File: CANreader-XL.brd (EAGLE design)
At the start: 99.8 x 49.8 mm, 101 parts, among them IC1 STM32F107RBT, IC2 TJA1055T/3, IC3 BD9G101G, IC4 LM1117IMPX-3.3, IC5 MCP2562-SOIC8, IC7 DP83848I, Q1 25MHz, SW1 SLEEP, SW2 TERM, U1 HC_05, X1 ST-USB-009A, X2 SWD, X3 CAN+GPIO, X4 UART

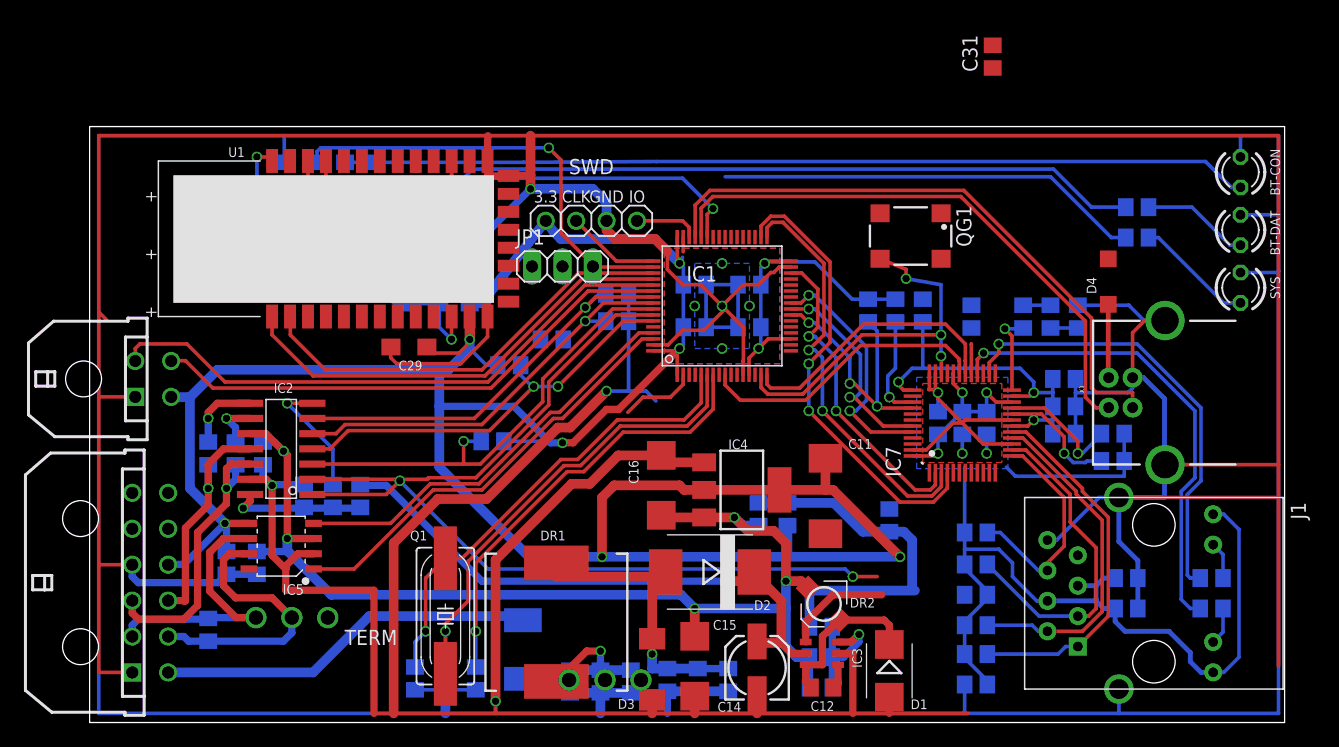
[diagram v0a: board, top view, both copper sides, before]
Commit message: Route attempt
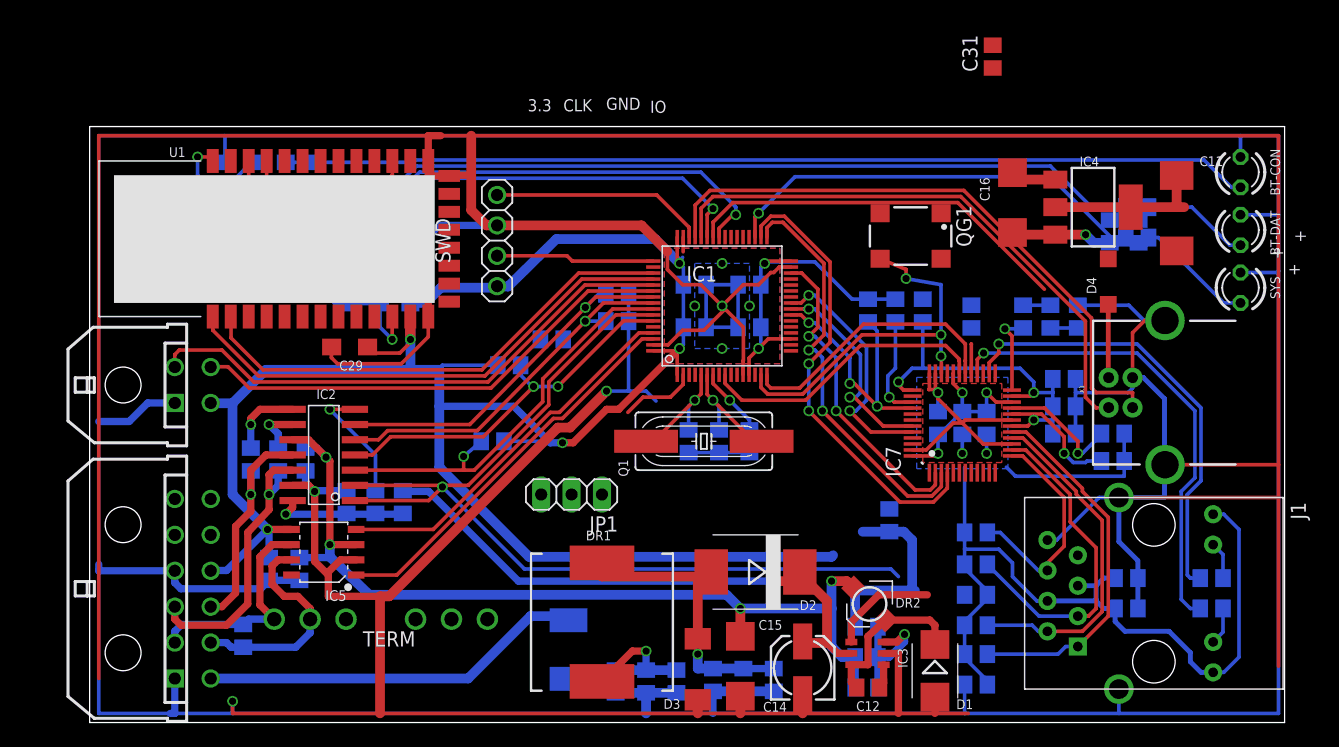
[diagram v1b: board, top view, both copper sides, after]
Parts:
- moved C11 37.7 mm to (90.8, 42.5)
- moved C16 37.7 mm to (77.1, 43.4)
- moved C17 37.7 mm to (85.2, 41.0)
- moved C18 37.7 mm to (87.6, 41.0)
- moved IC4 37.7 mm to (83.8, 43.1)
- moved C2 30.3 mm to (52.6, 23.5)
- moved C1 30.3 mm to (50.0, 23.5)
- moved C3 30.3 mm to (55.1, 23.5)
- moved Q1 26.1 mm to (51.3, 23.5), turned to 180 degrees
- moved JP1 19.1 mm to (40.3, 19.1), turned to 180 degrees
- moved SW1 13.8 mm to (30.2, 8.64)
- moved X2 8.05 mm to (34.0, 40.3), turned to 90 degrees
- moved C27 4.95 mm to (21.7, 35.9)
- moved C29 4.95 mm to (21.7, 31.4)
- moved R9 4.95 mm to (18.9, 45.8)
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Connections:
- net HC_KEY: now also IC1.41; no longer IC1.50
- net N$6: now also IC1.35; no longer IC1.41
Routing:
- net +3V3: track 346.0 -> 309.7 mm, vias 12 -> 10
- net USB_VBUS: track 6.15 -> 38.8 mm
- net NRST: track 36.7 -> 5.86 mm
- net GND: track 973.4 -> 942.6 mm, vias 12 -> 11
- net N$2: track 41.1 -> 10.5 mm
- net N$1: track 39.2 -> 10.5 mm
- net SWDIO: track 5.40 -> 18.0 mm
- net HC_KEY: track 36.9 -> 49.0 mm
- net +5V: track 94.0 -> 85.6 mm
- net N$15: track 0.00 -> 6.50 mm
- net SWCLK: track 7.83 -> 13.2 mm
- net N$10: track 74.6 -> 79.8 mm
- net UART4_TX: track 36.4 -> 41.5 mm
- net N$33: track 75.7 -> 80.8 mm
- net CAN2H: track 23.4 -> 18.4 mm
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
